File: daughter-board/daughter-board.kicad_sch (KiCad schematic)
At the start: 8 parts, among them J1 USB-C Connector, J2 Ribbon Connector, P1 IPOD_CONNECTOR_MALE, U1 AP2331SA-7

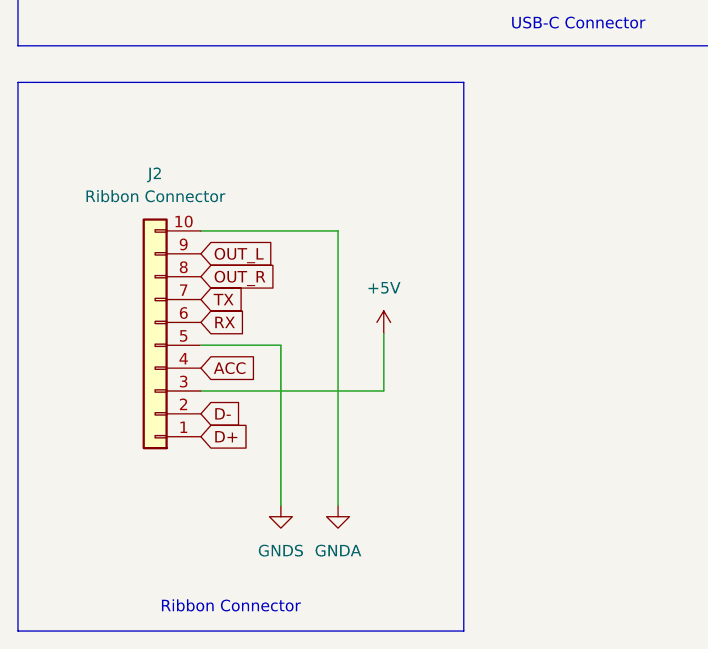
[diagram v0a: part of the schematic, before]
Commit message: Eh, not sure about this.
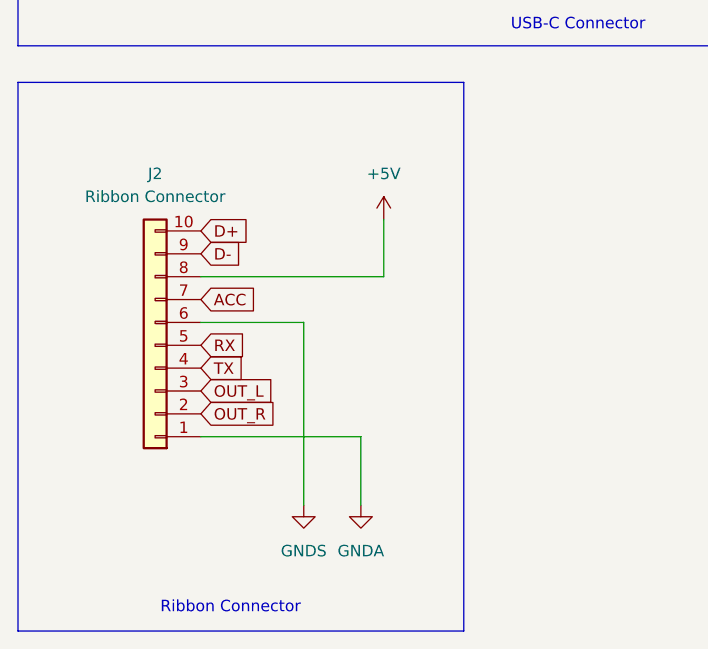
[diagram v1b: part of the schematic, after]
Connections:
- net +5V: now also J2.8 (Pin_8); no longer J2.3 (Pin_3)
- net ACC: now also J2.7 (Pin_7); no longer J2.4 (Pin_4)
- net D+: now also J2.10 (Pin_10); no longer J2.1 (Pin_1)
- net D-: now also J2.9 (Pin_9); no longer J2.2 (Pin_2)
- net GNDA: now also J2.1 (Pin_1); no longer J2.10 (Pin_10)
- net GNDS: now also J2.6 (Pin_6); no longer J2.5 (Pin_5)
- net OUT_L: now also J2.3 (Pin_3); no longer J2.9 (Pin_9)
- net OUT_R: now also J2.2 (Pin_2); no longer J2.8 (Pin_8)
- net RX: now also J2.5 (Pin_5); no longer J2.6 (Pin_6)
- net TX: now also J2.4 (Pin_4); no longer J2.7 (Pin_7)
